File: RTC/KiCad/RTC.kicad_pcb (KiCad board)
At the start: 2 copper layers, 35 x 12 mm, 5 parts, among them J1 Conn_01x04, J2 Conn_01x04, J3 Conn_01x04

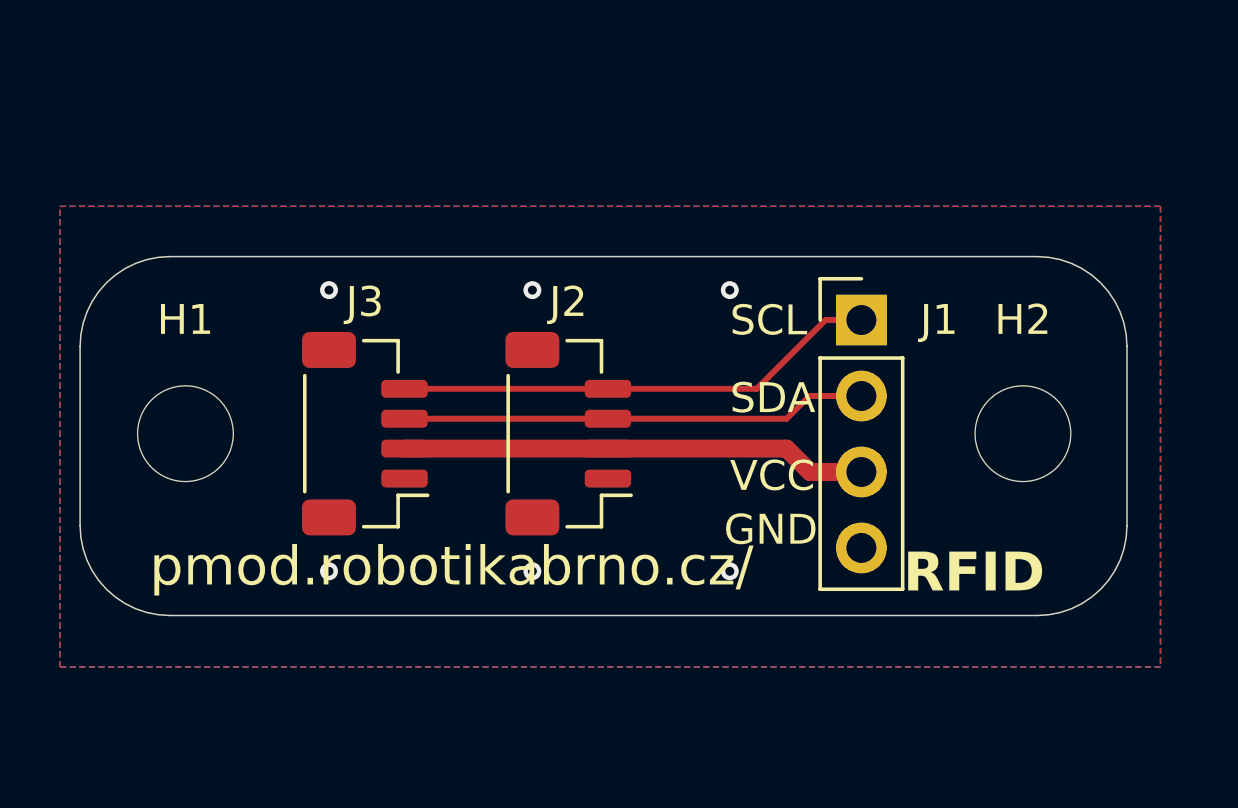
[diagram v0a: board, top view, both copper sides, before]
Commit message: Deployed d972a79 with MkDocs version: 1.6.0
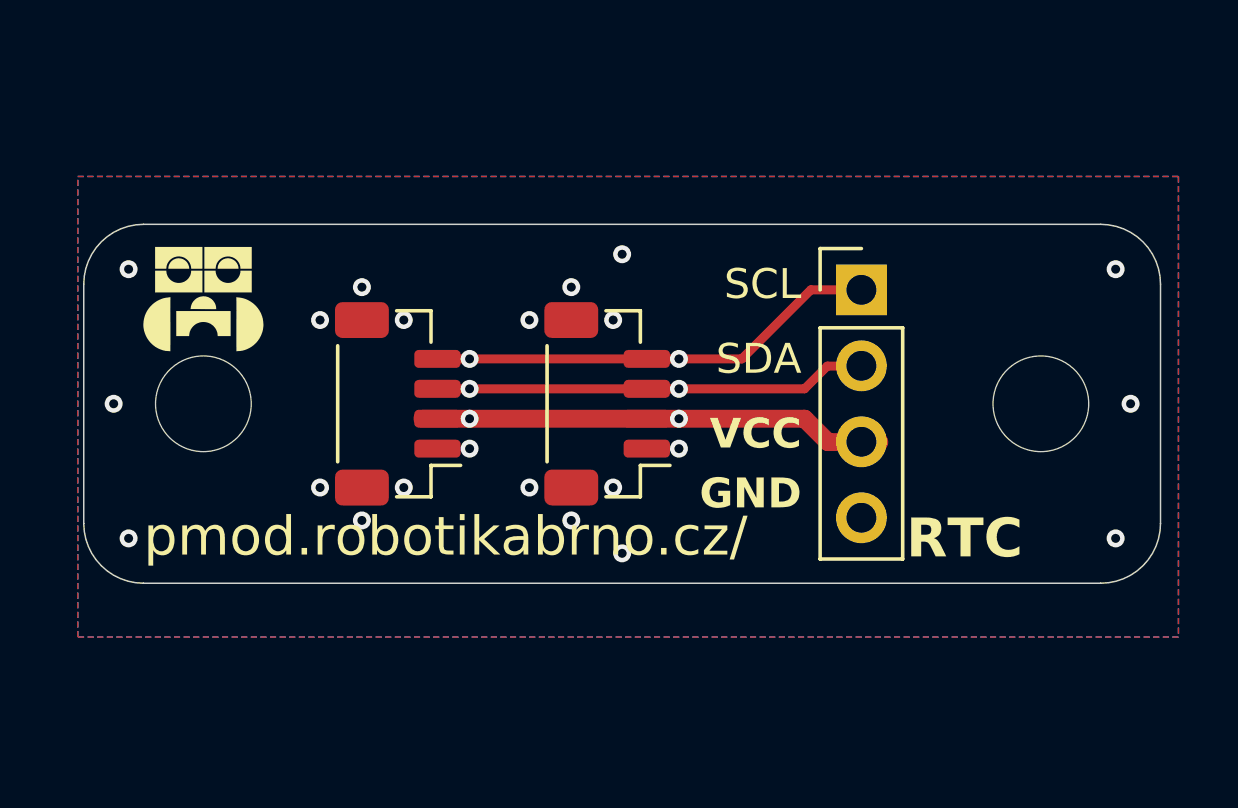
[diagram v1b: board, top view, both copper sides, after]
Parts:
- H1, H2: footprint MountingHole:MountingHole_3.2mm_M3_DIN965 -> MountingHole:MountingHole_3.2mm_M3
- moved J2 1.64 mm to (144.5, 79.0)
- moved J3 1.49 mm to (137.5, 79.0)
- moved H1 1.17 mm to (131.0, 79.0)
- moved H2 1.17 mm to (159.0, 79.0)
- moved J1 1.01 mm to (153.0, 75.2)
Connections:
- J2 pad MP: (no net) -> GND
- J3 pad MP: (no net) -> GND
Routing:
- net Net-(J1-Pin_1): vias 0 -> 2
- net Net-(J1-Pin_2): vias 0 -> 2
- net VCC: vias 0 -> 2
- net GND: vias 6 -> 22
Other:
- board size 35 x 12 mm -> 36 x 12 mm
- board text added: "12mm"
- board text added: "36mm"
- board text added: "RTC"
- board text removed: "RFID"

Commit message: Deployed 2be6636 with MkDocs version: 1.6.0
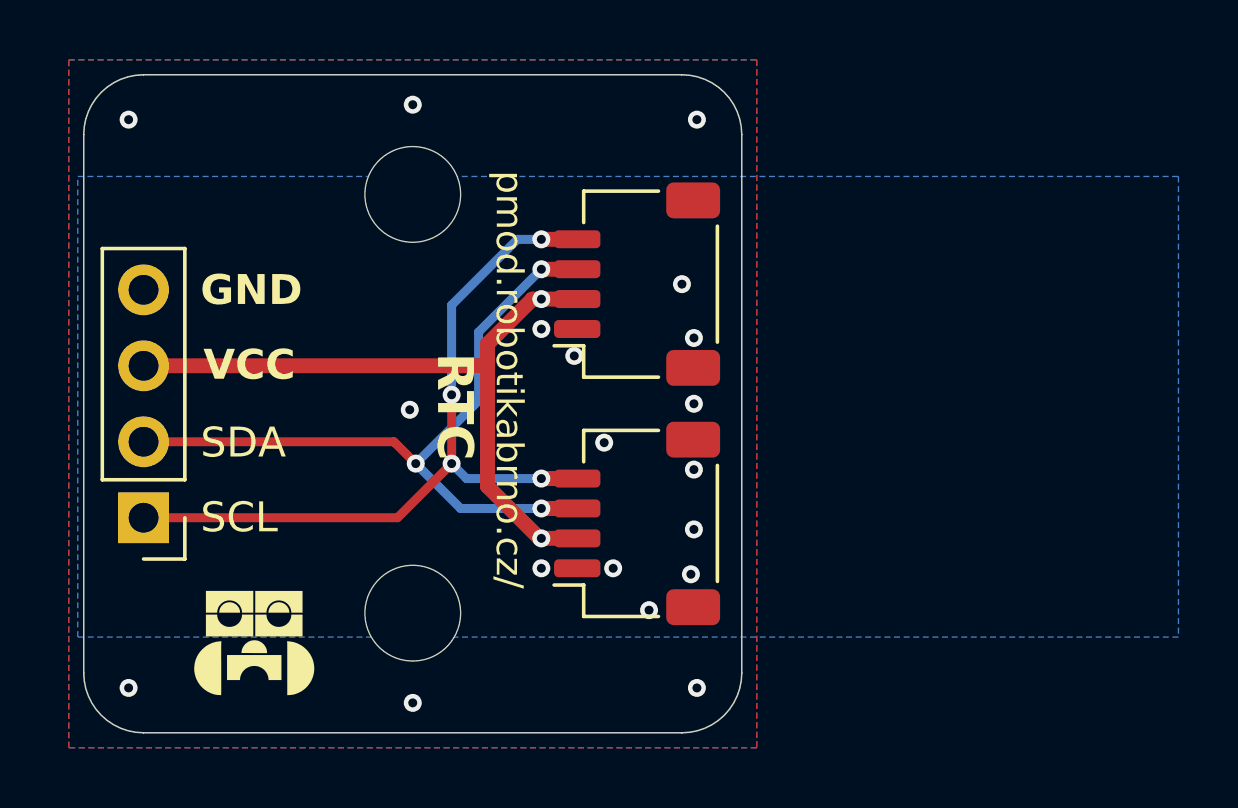
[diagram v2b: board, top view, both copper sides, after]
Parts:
- J2, J3: value Conn_01x04 -> Conn_01x04_Pin; footprint Connector_JST:JST_SH_BM04B-SRSS-TB_1x04-1MP_P1.00mm_Vertical -> Connector_JST:JST_SH_SM04B-SRSS-TB_1x04-1MP_P1.00mm_Horizontal
- moved J1 25.2 mm to (129.0, 82.8), turned to 180 degrees
- moved H2 22.1 mm to (138.0, 72.0)
- moved H1 9.90 mm to (138.0, 86.0)
- moved J3 8.94 mm to (145.5, 83.0)
- moved J2 4.12 mm to (145.5, 75.0)
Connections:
- net Net-(J1-Pin_1) renamed /SCL
- net Net-(J1-Pin_2) renamed /SDA
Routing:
- net /SCL: track 16.2 -> 25.9 mm, vias 2 -> 4
- net /SDA: track 15.6 -> 24.9 mm, vias 2 -> 3
- net VCC: track 15.6 -> 23.6 mm
- net GND: vias 22 -> 19
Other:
- board size 36 x 12 mm -> 22 x 22 mm
- board text added: "22mm"
- board text removed: "12mm"
- board text removed: "36mm"
